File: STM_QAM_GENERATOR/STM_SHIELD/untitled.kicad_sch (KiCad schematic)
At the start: 1 part, among them U1 NUCLEO-F446RE

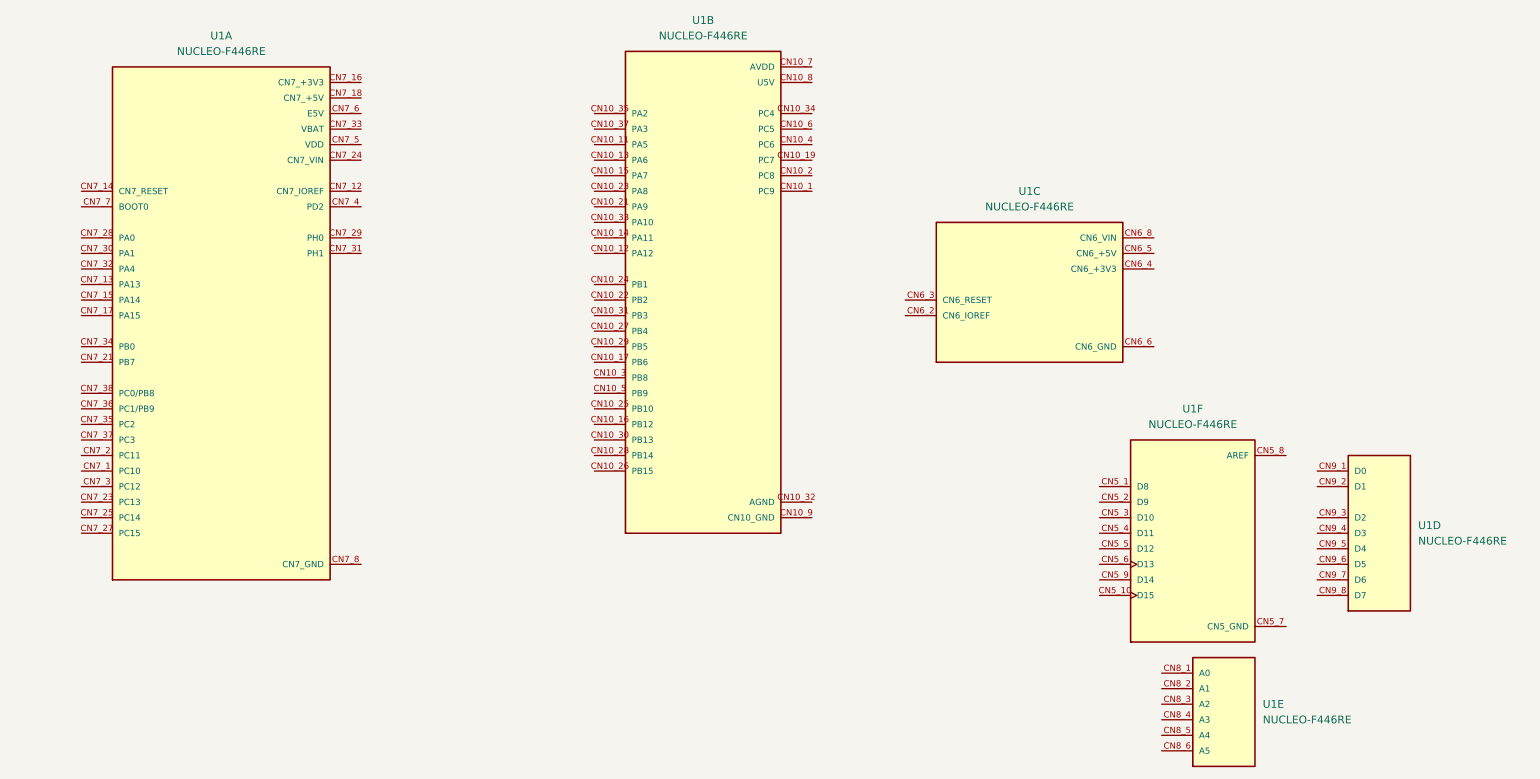
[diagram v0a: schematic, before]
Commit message: STM_SHIELD_DONE
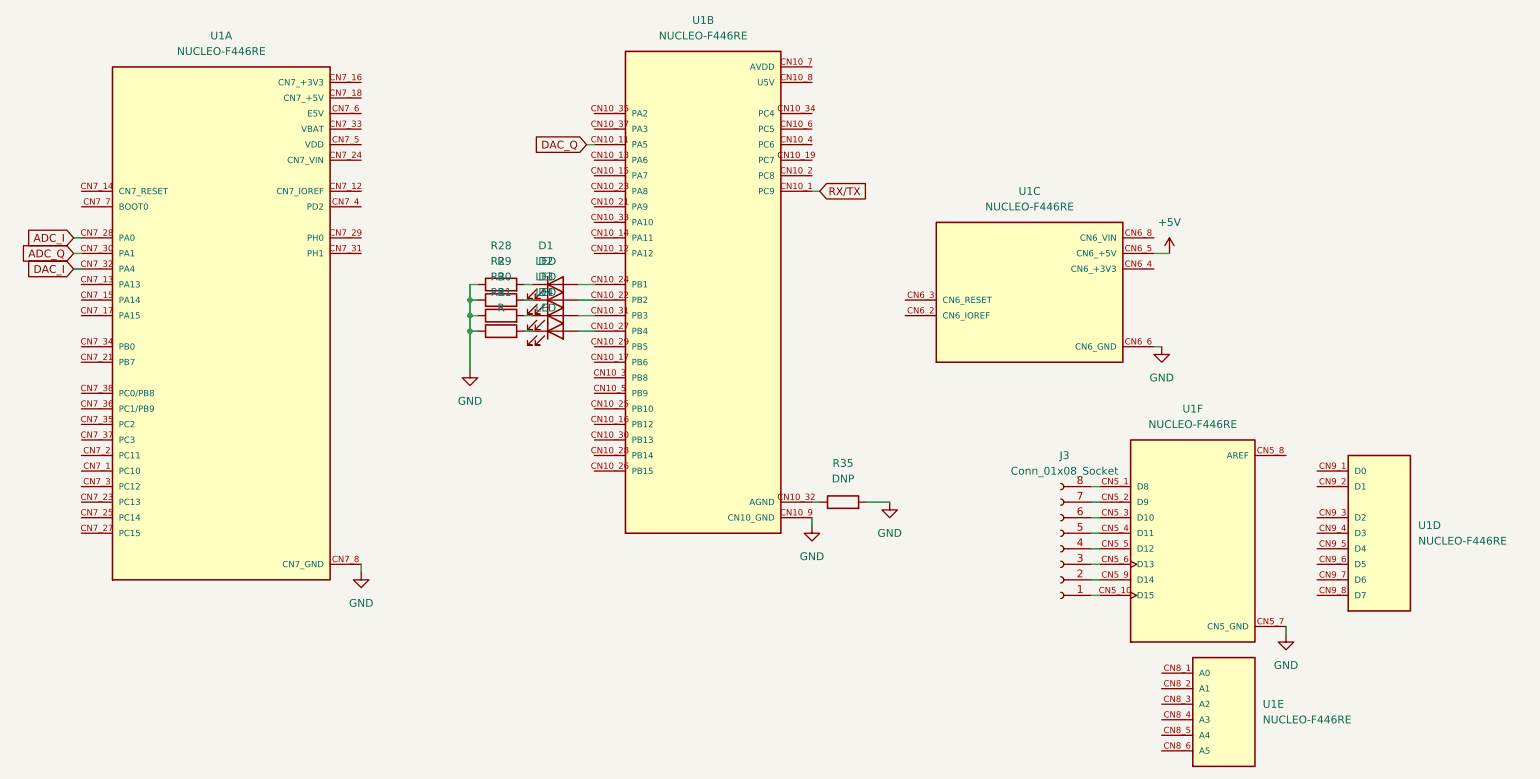
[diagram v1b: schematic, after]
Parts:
- added D1, D2, D3, D4: LED, LED_SMD:LED_0603_1608Metric_Pad1.05x0.95mm_HandSolder, symbol Device:LED
- added J3: Conn_01x08_Socket, Connector_PinSocket_2.54mm:PinSocket_1x08_P2.54mm_Vertical, symbol Connector:Conn_01x08_Socket
- added R28, R29, R30, R31: R, Resistor_SMD:R_0603_1608Metric_Pad0.98x0.95mm_HandSolder, symbol Device:R
- added R35: DNP, Resistor_SMD:R_0603_1608Metric_Pad0.98x0.95mm_HandSolder, symbol Device:R
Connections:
- net CN6_GND is gone; now on net CN10_GND: U1.CN6_6 (CN6_GND), U1.CN6_7 (CN6_GND)
- net CN7_GND is gone; now on net CN10_GND: U1.CN7_19 (CN7_GND), U1.CN7_20 (CN7_GND), U1.CN7_22 (CN7_GND), U1.CN7_8 (CN7_GND)
- net CN10_GND: now also U1.CN5_7 (CN5_GND), R28.1, R29.1, R30.1, R31.1, R35.2
- net at U1.CN5_1 (D8): now also J3.8 (Pin_8)
- net at U1.CN5_10 (D15): now also J3.1 (Pin_1)
- net at U1.CN5_2 (D9): now also J3.7 (Pin_7)
- net at U1.CN5_3 (D10): now also J3.6 (Pin_6)
- net at U1.CN5_4 (D11): now also J3.5 (Pin_5)
- net at U1.CN5_5 (D12): now also J3.4 (Pin_4)
- net at U1.CN5_6 (D13): now also J3.3 (Pin_3)
- net at U1.CN5_9 (D14): now also J3.2 (Pin_2)
- net +5V: now reaches U1.CN6_5 (CN6_+5V)
- net RX/TX: now reaches U1.CN10_1 (PC9)
- net DAC_Q: now reaches U1.CN10_11 (PA5)
- net at U1.CN10_22 (PB2): now also D2.2 (A)
- net at U1.CN10_24 (PB1): now also D1.2 (A)
- net at U1.CN10_27 (PB4): now also D4.2 (A)
- net at U1.CN10_31 (PB3): now also D3.2 (A)
- net at U1.CN10_32 (AGND): now also R35.1
- net ADC_I: now reaches U1.CN7_28 (PA0)
- net ADC_Q: now reaches U1.CN7_30 (PA1)
- net DAC_I: now reaches U1.CN7_32 (PA4)
- new net: D4.1 (K), R31.2
- new net: D2.1 (K), R29.2
- new net: D3.1 (K), R30.2
- new net: D1.1 (K), R28.2

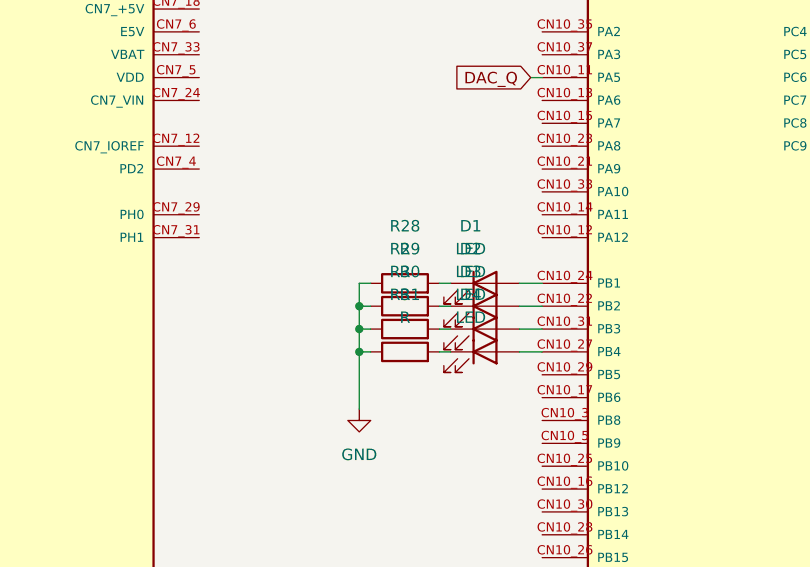
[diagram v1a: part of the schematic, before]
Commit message: Added values to schematics
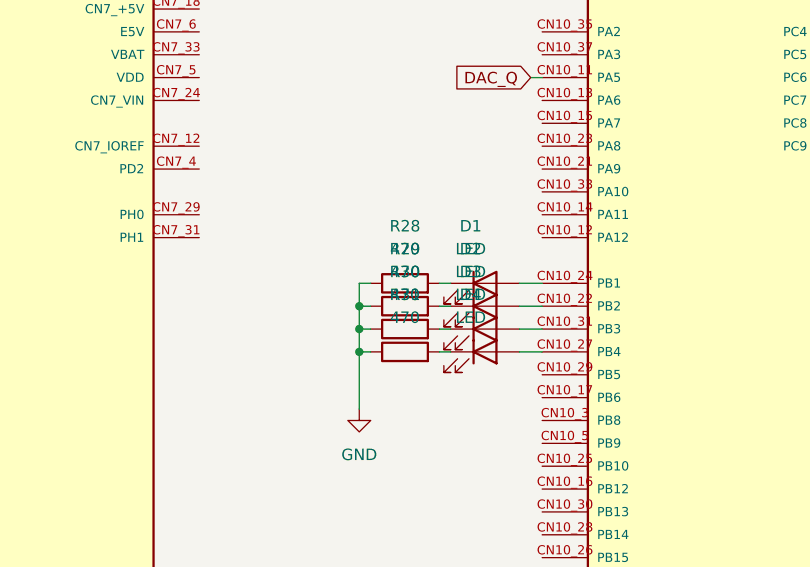
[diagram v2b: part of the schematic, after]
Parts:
- R28, R29, R30, R31: value R -> 470
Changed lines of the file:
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@@
 			)
 		)
-		(property "Value" "R"
+		(property "Value" "470"
 			(at 114.3 82.55 90)
 			(effects
@@
 			)
 		)
-		(property "Value" "R"
+		(property "Value" "470"
 			(at 114.3 77.47 90)
 			(effects
@@
 			)
 		)
-		(property "Value" "R"
+		(property "Value" "470"
 			(at 114.3 74.93 90)
 			(effects
@@
 			)
 		)
-		(property "Value" "R"
+		(property "Value" "470"
 			(at 114.3 80.01 90)
 			(effects
